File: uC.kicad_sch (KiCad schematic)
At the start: 21 parts, among them J201 5023860270, J202 Conn_01x05, J203 Conn_01x04, J204 Conn_01x04, U201 STM32G431KBT6, Y201 ECS-2520MV-xxx-xx

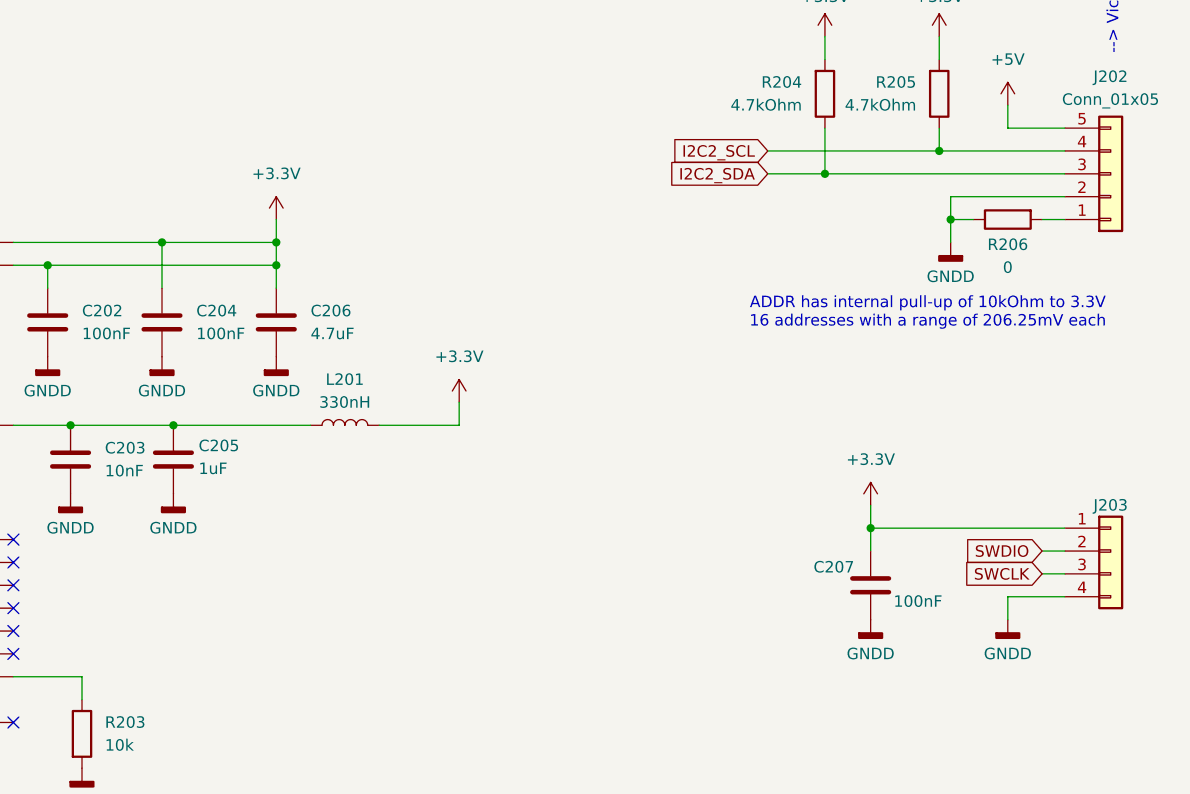
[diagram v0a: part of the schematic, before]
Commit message: progress on layout in general, minor tweaks to schemas
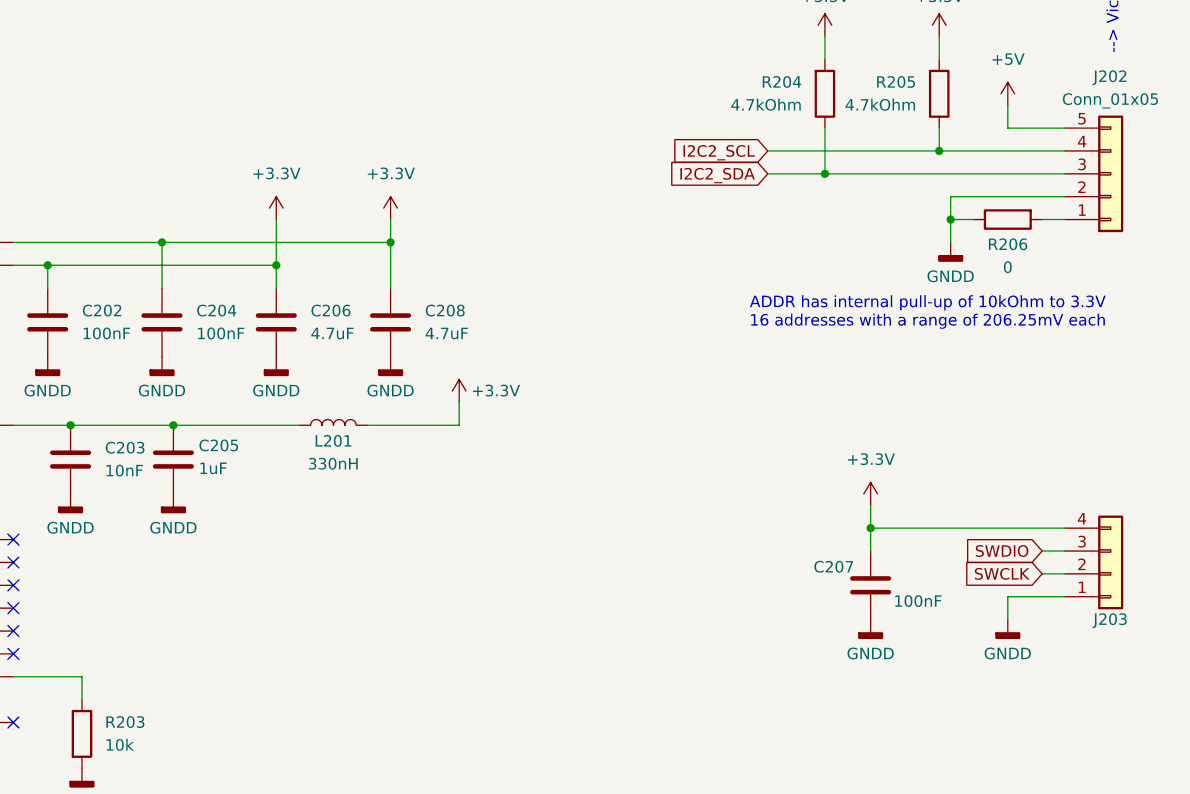
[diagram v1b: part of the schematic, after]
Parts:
- added C208: 4.7uF, Capacitor_SMD:C_0603_1608Metric, symbol Device:C
- C201, C202, C203: footprint Capacitor_SMD:C_0805_2012Metric -> Capacitor_SMD:C_0603_1608Metric
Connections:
- net +3.3V: now also J203.4 (Pin_4), C208.1; no longer J203.1 (Pin_1)
- net GNDA: now also J203.1 (Pin_1), C208.2; no longer J203.4 (Pin_4)
- net SWCLK: now also J203.2 (Pin_2); no longer J203.3 (Pin_3)
- net SWDIO: now also J203.3 (Pin_3); no longer J203.2 (Pin_2)
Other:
- moved on the sheet: L201
